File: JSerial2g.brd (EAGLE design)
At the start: 50 x 50 mm, 59 parts, among them CN1 USBMOLEX, IC1 FT232RL, Q1 2N3904SOT23, Q2 2N3904SOT23, Q3 BC547, Q4 BC547, X1 RJ45-8X

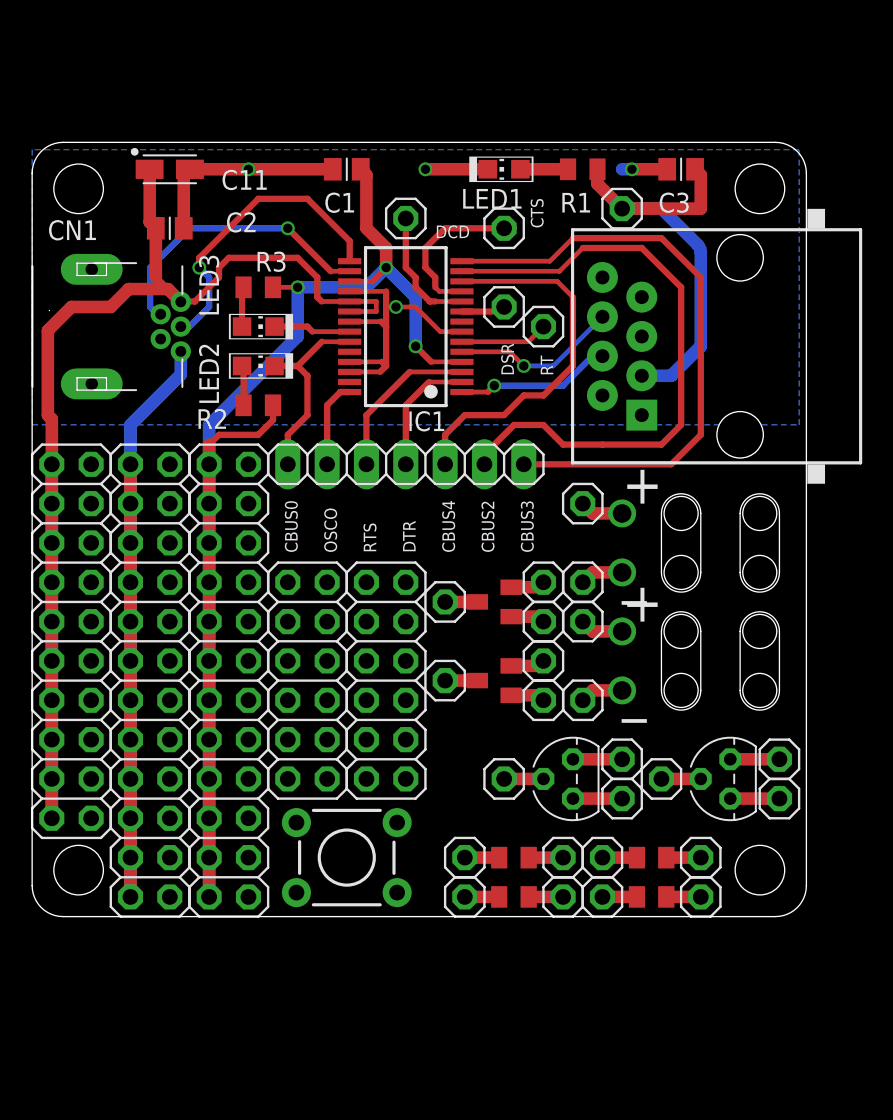
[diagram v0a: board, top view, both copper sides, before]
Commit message: JSerial 2G in progress
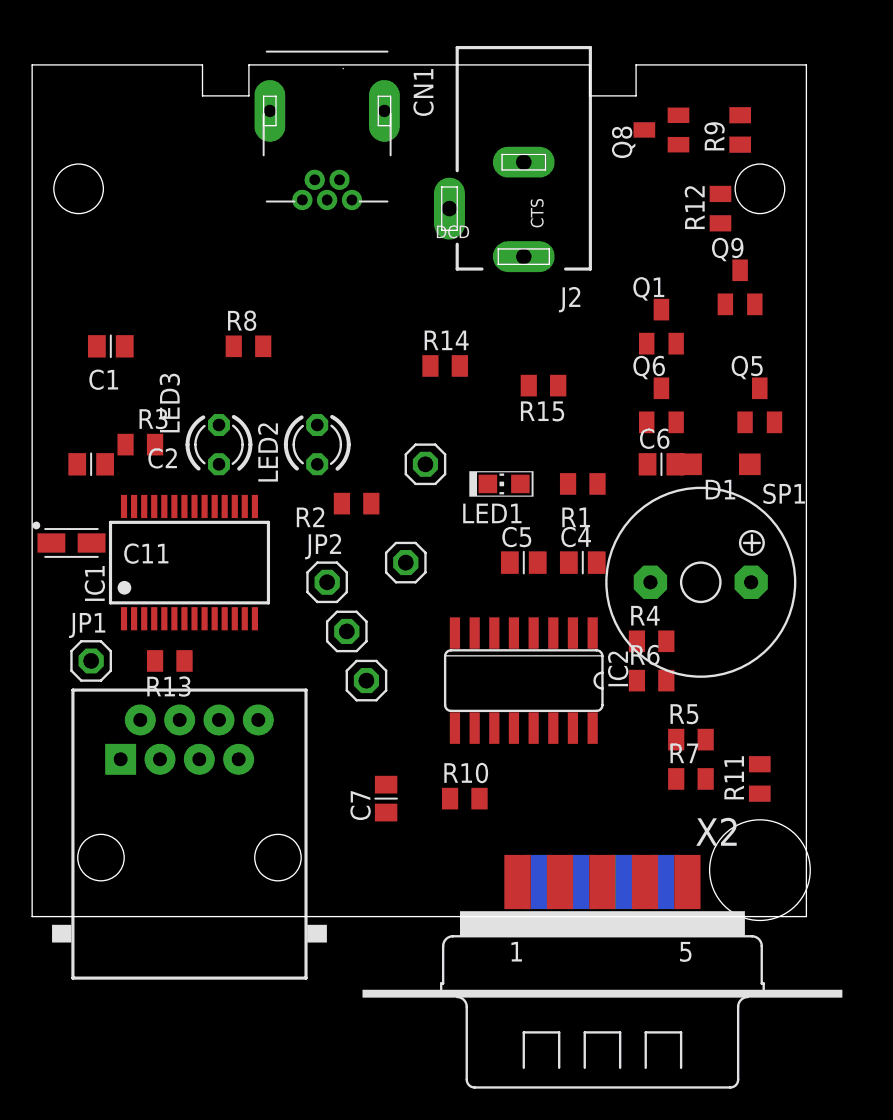
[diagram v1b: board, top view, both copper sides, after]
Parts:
- removed C3: 0.47 uF, ipc-7351-capacitor:CAPC2012X145AN
- removed J1, J4: (no value), jlab:FLEX-POWER
- removed JP10, JP11, JP12, JP13, JP14, JP15, JP16, JP17, JP18, JP19, JP20, JP21, JP22, JP23, JP24, JP25, JP26, JP27, JP28, JP35, JP4, JP5, JP6, JP7, JP9: (no value), pinhead:1X01
- removed JP29: (no value), pinhead:2X10
- removed JP3: (no value), pinhead:2X12
- removed JP30: (no value), pinhead:2X06
- removed JP8: (no value), pinhead:1X07
- removed Q2: 2N3904SOT23, transistor-npn:SOT23-BEC
- removed Q3, Q4: BC547, transistor-npn:TO92
- removed S1: DT5X6, jlab:TACTILE-PTH
- added C4, C5, C6, C7: 0.1uF, ipc-7351-capacitor:CAPC2012X145AN
- added D1: 1N4148, diode:SOD123
- added IC2: MAX3232CSE, maxim:SO16
- added J2: DCJ0202, con-jack:DCJ0202
- added Q5, Q6, Q8: BC857BSMD, transistor-pnp:SOT23-BEC
- added Q9: 2N3904SOT23, transistor-npn:SOT23-BEC
- added R10, R12, R14: 1K, ipc-7351-resistor:RESC2012X70N
- added R11, R13, R9: 10K, ipc-7351-resistor:RESC2012X70N
- added R15: 100, ipc-7351-resistor:RESC2012X70N
- added R8: 4.7K, ipc-7351-resistor:RESC2012X70N
- added SP1: KSS1201, buzzer:KSS1201
- added X2: (no value), jlab:M09D
- JP1: device pinhead:2X06 -> pinhead:1X01
- JP2: device pinhead:2X12 -> pinhead:1X01
- LED2, LED3: device jlab:CHIP-LED0805 -> jlab:LED3MM
- R2, R3: value 270 R -> 470
- R4, R7: value 270 R -> 1K
- R5, R6: value 270 R -> 10K
- moved X1 48.5 mm to (10.2, 3.81), turned to 0 degrees
- moved JP33 26.9 mm to (20.3, 18.4)
- moved CN1 26.1 mm to (19.1, 55.9), turned to 180 degrees
- moved JP34 25.6 mm to (21.6, 15.2)
- moved Q1 25.3 mm to (40.6, 38.1), turned to 0 degrees
- moved C11 25.0 mm to (2.54, 24.1)
- moved JP31 22.5 mm to (24.1, 22.9)
- moved IC1 20.7 mm to (10.2, 22.9), turned to 0 degrees
- moved LED1 20.3 mm to (30.5, 27.9)
- moved R1 20.3 mm to (35.6, 27.9)
- moved JP1 19.1 mm to (3.81, 16.5), turned to 0 degrees
- moved C1 19.1 mm to (5.08, 36.8)
- moved C2 16.1 mm to (3.81, 29.2)
- moved R4 14.0 mm to (40.0, 17.8), turned to 0 degrees
- moved R6 14.0 mm to (40.0, 15.2)
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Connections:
- net RT renamed RI
- removed net N$23: JP22.1, R4.1
- removed net N$24: JP14.1, Q3.3
- removed net N$25: JP18.1, Q4.3
- removed net N$26: JP19.1, Q4.1
- removed net N$27: JP20.1, Q3.1
- removed net N$28: JP23.1, R5.1
- removed net N$29: JP24.1, R7.1
- removed net N$30: JP13.1, Q1.C
- removed net N$31: JP15.1, Q1.E
- removed net N$32: JP17.1, Q2.C
- removed net N$33: JP16.1, Q2.E
- removed net N$34: JP25.1, R7.2
- removed net N$35: JP26.1, R5.2
- removed net N$36: JP27.1, R4.2
- removed net N$37: JP28.1, R6.2
- removed net OSCO: IC1.28, JP8.2
- new net N$13: IC2.13, X2.2
- new net N$14: J2.1, Q8.C
- new net N$15: Q5.B, R5.1, R7.2
- new net N$16: Q6.B, R4.2, R6.1
- new net N$17: Q9.B, R10.2, R11.2
- new net N$2: C4.1, IC2.3
- new net N$7: C4.2, IC2.1
- new net N$8: C5.1, IC2.5
- new net TX_TTL_INV: IC1.5, Q5.C, Q6.C, R8.2
- new net TX_TTL_MAXIM: IC2.12, R4.1
- net +3V3: now also C6.2, IC2.16, Q5.E, Q6.E, R13.2, R5.2, R6.2; no longer JP3.10, JP3.12, JP3.14, JP3.16, JP3.18, JP3.2, JP3.20, JP3.22, JP3.24, JP3.4, JP3.6, JP3.8
- net +5V: now also Q8.E, R15.2, R9.2; no longer JP29.10, JP29.12, JP29.14, JP29.16, JP29.18, JP29.2, JP29.20, JP29.4, JP29.6, JP29.8
- net CBUS0: now also LED2.K; no longer JP8.1, LED2.C
- net CBUS1: now also LED3.K; no longer LED3.C
- net CBUS2: now also R10.1; no longer JP8.6
- net CBUS3: now also JP33.1; no longer JP8.7
- net CBUS4: now also JP2.1; no longer JP8.5
- net DCD: now also J2.2, R13.1; no longer JP33.1
- net DTR: now also JP1.1; no longer JP8.4
- net GND: now also C7.2, IC2.15, J2.3, Q1.E, Q9.E, R11.1, R8.1, X2.5; no longer C3.1, JP2.10, JP2.12, JP2.14, JP2.16, JP2.18, JP2.2, JP2.20, JP2.22, JP2.24, JP2.4, JP2.6, JP2.8
- net N$10: now also C6.1, IC2.2; no longer J1.2, JP5.1
- net N$11: now also C7.1, IC2.6; no longer J4.1, JP6.1
- net N$12: now also IC2.14, X2.3; no longer J4.2, JP7.1
- net N$18: now also Q9.C, R12.1; no longer JP9.1, Q3.2
- net N$19: now also Q8.B, R12.2, R9.1; no longer JP10.1, Q4.2
- net N$20: now also Q1.B, R14.2; no longer JP12.1, Q2.B
- net N$21: now also D1.A, Q1.C, SP1.-; no longer JP11.1, Q1.B
- net N$22: now also D1.C, R15.1, SP1.+; no longer JP21.1, R6.1
- net N$9: now also C5.2, IC2.4; no longer J1.1, JP4.1
- net RTS: now also R14.1; no longer JP8.3
- net RX_TTL: now also IC2.11
- net TX_TTL: now also R7.1; no longer IC1.5
- net VCC: no longer C3.2, JP35.1
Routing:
- net GND: track 133.4 -> 0.00 mm, vias 4 -> 0
- net +3V3: track 103.9 -> 0.00 mm, vias 3 -> 0
- net +5V: track 91.2 -> 0.00 mm
- net CBUS2: track 39.9 -> 0.00 mm
- net CBUS3: track 39.5 -> 0.00 mm
- net VCC: track 28.0 -> 0.00 mm
- net CBUS4: track 24.0 -> 0.00 mm
- net N$3: track 19.5 -> 0.00 mm, vias 1 -> 0
- net N$4: track 18.5 -> 0.00 mm, vias 1 -> 0
- net CBUS0: track 12.6 -> 0.00 mm
- net CTS: track 10.9 -> 0.00 mm
- net TX_TTL: track 10.8 -> 0.00 mm, vias 1 -> 0
- net RTS: track 10.5 -> 0.00 mm
- net RX_TTL: track 10.0 -> 0.00 mm, vias 1 -> 0
- net DCD: track 8.08 -> 0.00 mm
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- removed copper zone on layer 16, net GND
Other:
- board size 50 x 50 mm -> 50 x 55 mm
- board text removed: "CBUS0"
- board text removed: "CBUS2"
- board text removed: "CBUS3"
- board text removed: "CBUS4"
- board text removed: "DSR"
- board text removed: "DTR"
- board text removed: "OSCO"
- board text removed: "RT"
- board text removed: "RTS"

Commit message: Work in progress
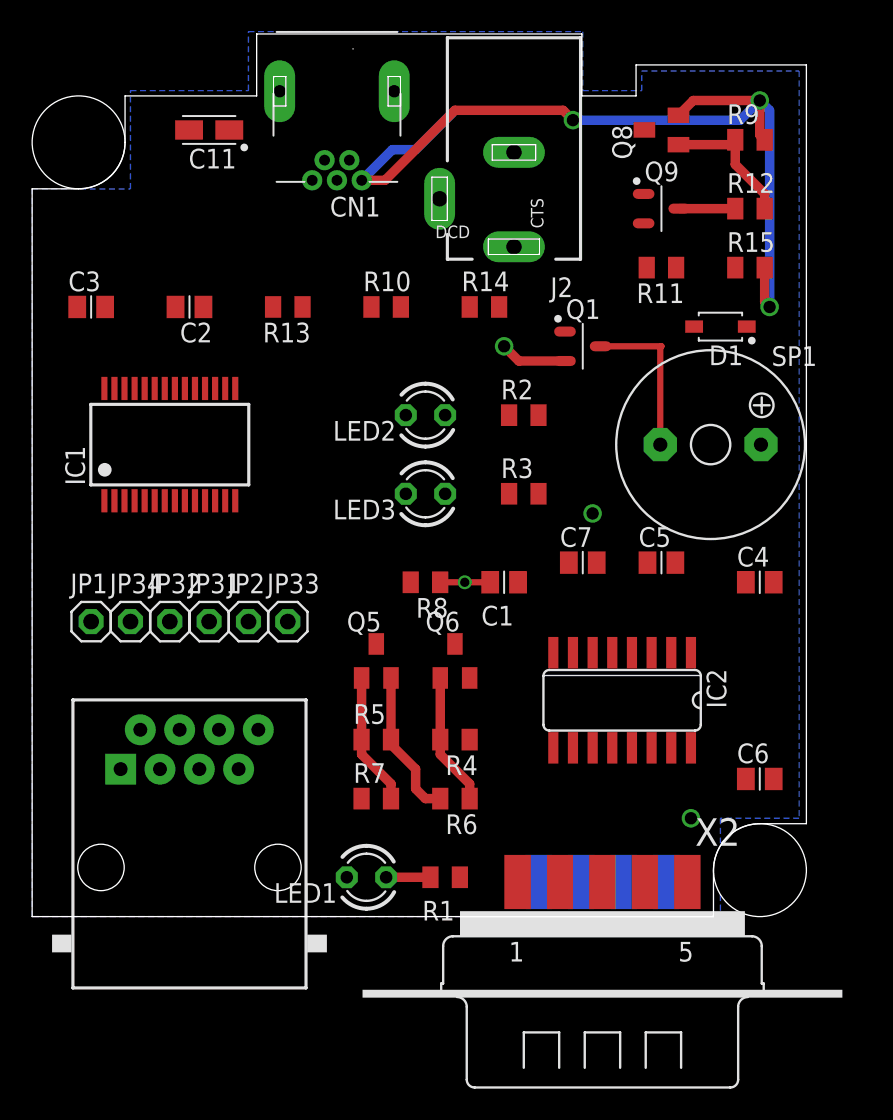
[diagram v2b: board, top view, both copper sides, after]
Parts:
- added C3: 0.1 uF, ipc-7351-capacitor:CAPC2012X145AN
- D1: device diode:SOD123 -> ipc-7351-diode:SOD3718X135N
- LED1: device jlab:CHIP-LED0805 -> jlab:LED3MM
- Q1: value 2N3904SOT23 -> 2N3904 SOT23; device transistor-npn:SOT23-BEC -> ipc-7351-transistor:SOT95P280X135-3N
- Q9: value 2N3904SOT23 -> 2N3904; device transistor-npn:SOT23-BEC -> ipc-7351-transistor:SOT95P280X135-3N
- moved R11 33.6 mm to (40.6, 41.9), turned to 180 degrees
- moved R10 32.2 mm to (22.9, 39.4)
- moved Q5 29.8 mm to (22.2, 16.5)
- moved C1 29.6 mm to (30.5, 21.6)
- moved C11 28.1 mm to (11.4, 50.8), turned to 180 degrees
- moved LED1 26.9 mm to (21.6, 2.54), turned to 180 degrees
- moved R1 26.9 mm to (26.7, 2.54)
- moved R3 25.0 mm to (31.8, 27.3)
- moved R13 24.1 mm to (16.5, 39.4)
- moved C6 21.3 mm to (47.0, 8.89)
- moved Q6 21.2 mm to (27.3, 16.5)
- moved R7 20.4 mm to (22.2, 7.62)
- moved R5 20.3 mm to (22.2, 11.4)
- moved C7 19.8 mm to (35.6, 22.9), turned to 0 degrees
- moved JP32 19.4 mm to (8.89, 19.1)
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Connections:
- net +3V3: now also C3.2
- net GND: now also C3.1, LED1.K, Q1.2, Q9.2; no longer LED1.C, Q1.E, Q9.E
- net N$17: now also Q9.1; no longer Q9.B
- net N$18: now also Q9.3; no longer Q9.C
- net N$20: now also Q1.1; no longer Q1.B
- net N$21: now also Q1.3; no longer Q1.C
- net N$22: now also D1.K; no longer D1.C
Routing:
- net +5V: track 0.00 -> 60.8 mm, vias 0 -> 3
- net N$21: track 0.00 -> 10.3 mm
- net +3V3: track 0.00 -> 9.67 mm
- net N$19: track 0.00 -> 9.03 mm
- net N$15: track 0.00 -> 8.58 mm
- net N$16: track 0.00 -> 8.58 mm
- net GND: track 0.00 -> 7.55 mm, vias 0 -> 4
- net N$18: track 0.00 -> 3.62 mm
- net N$1: track 0.00 -> 2.86 mm
- added copper zone on layer 16, net GND
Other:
- board size 50 x 55 mm -> 50 x 57 mm
